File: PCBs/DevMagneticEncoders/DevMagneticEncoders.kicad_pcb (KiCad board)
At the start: 2 copper layers, 55 x 56 mm, 23 parts, among them J1 Conn_01x06_Male, J2 Conn_01x06_Male, J3 Screw_Terminal_01x02, J4 Conn_02x03_Odd_Even, J5 Conn_02x03_Odd_Even, J6 Conn_01x06_Male, J7 Conn_01x04_Male, J8 Conn_01x04_Male, U1 AZ1117-3.3, U2 ESP32-S2-WROOM

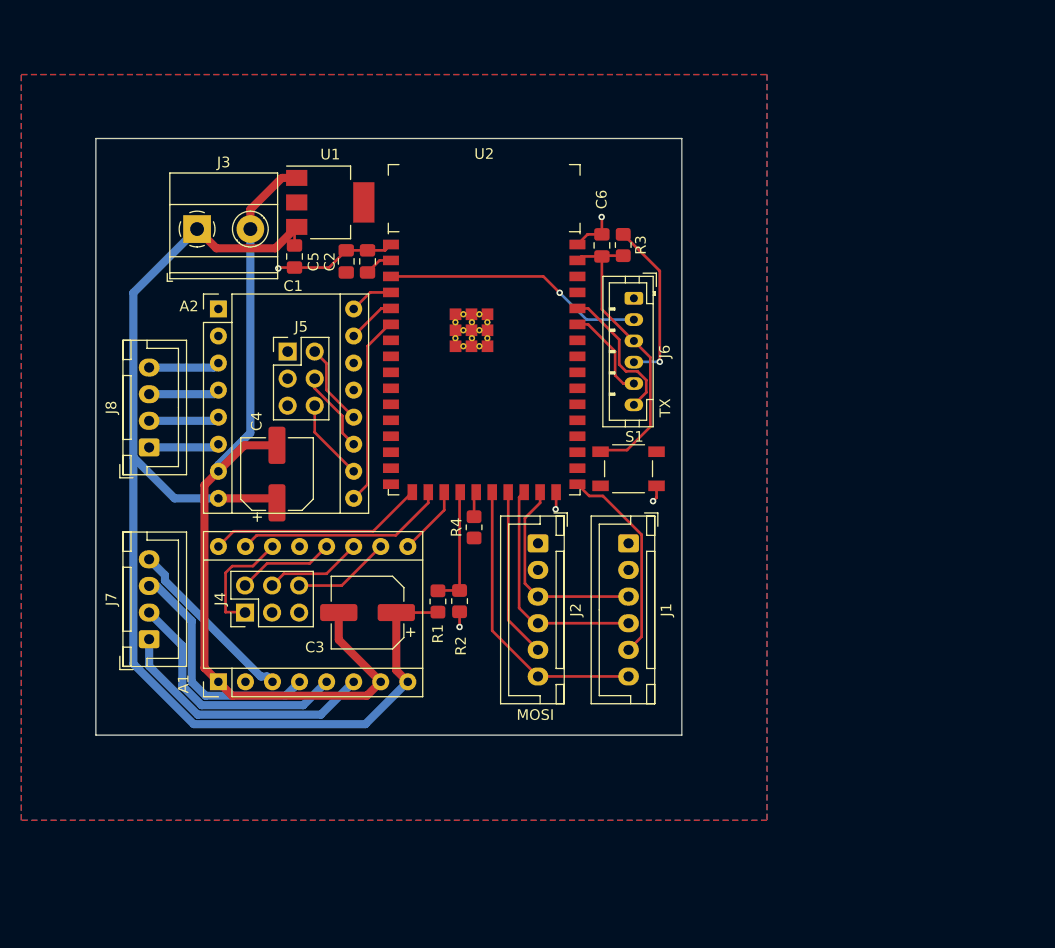
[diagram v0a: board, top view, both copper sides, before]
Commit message: 5 stepper board
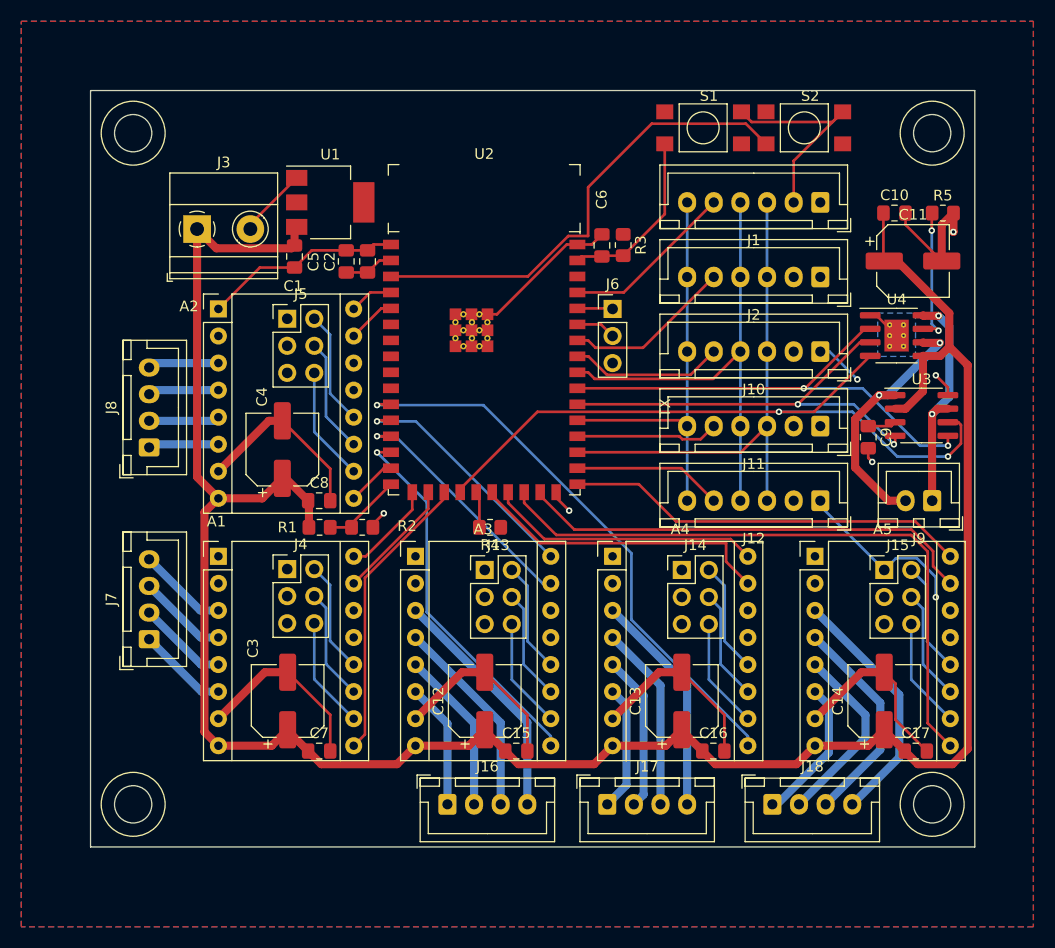
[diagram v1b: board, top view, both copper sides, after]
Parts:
- added A3: Pololu_Breakout_DRV8825, Module:Pololu_Breakout-16_15.2x20.3mm, F.Cu at (92.0, 95.2)
- added A4: Pololu_Breakout_DRV8825, Module:Pololu_Breakout-16_15.2x20.3mm, F.Cu at (110.5, 95.2)
- added A5: Pololu_Breakout_DRV8825, Module:Pololu_Breakout-16_15.2x20.3mm, F.Cu at (129.5, 95.2)
- added C10: 0.1U, Capacitor_SMD:C_0805_2012Metric_Pad1.18x1.45mm_HandSolder, F.Cu at (137.0, 63.0)
- added C11: 100U, Capacitor_SMD:CP_Elec_6.3x7.7, F.Cu at (138.7, 67.5)
- added C12: 100u, Capacitor_SMD:CP_Elec_6.3x7.7, F.Cu at (98.5, 108.8)
- added C13: 100u, Capacitor_SMD:CP_Elec_6.3x7.7, F.Cu at (117.0, 108.8)
- added C14: 100u, Capacitor_SMD:CP_Elec_6.3x7.7, F.Cu at (136.0, 108.8)
- added C15: 0.1u, Capacitor_SMD:C_0805_2012Metric_Pad1.18x1.45mm_HandSolder, F.Cu at (101.5, 113.5)
- added C16: 0.1u, Capacitor_SMD:C_0805_2012Metric_Pad1.18x1.45mm_HandSolder, F.Cu at (120.0, 113.5)
- added C17: 0.1u, Capacitor_SMD:C_0805_2012Metric_Pad1.18x1.45mm_HandSolder, F.Cu at (139.0, 113.5)
- added C7: 0.1u, Capacitor_SMD:C_0805_2012Metric_Pad1.18x1.45mm_HandSolder, F.Cu at (83.0, 113.5)
- added C8: 0.1u, Capacitor_SMD:C_0805_2012Metric_Pad1.18x1.45mm_HandSolder, F.Cu at (83.0, 90.0)
- added C9: 1U, Capacitor_SMD:C_0805_2012Metric_Pad1.18x1.45mm_HandSolder, F.Cu at (134.5, 84.0)
- added J10: Conn_01x06_Male, Connector_JST:JST_XH_B6B-XH-A_1x06_P2.50mm_Vertical, F.Cu at (130.0, 76.0)
- added J11: Conn_01x06_Male, Connector_JST:JST_XH_B6B-XH-A_1x06_P2.50mm_Vertical, F.Cu at (130.0, 83.0)
- added J12: Conn_01x06_Male, Connector_JST:JST_XH_B6B-XH-A_1x06_P2.50mm_Vertical, F.Cu at (130.0, 90.0)
- added J13: Conn_02x03_Odd_Even, Connector_PinHeader_2.54mm:PinHeader_2x03_P2.54mm_Vertical, F.Cu at (98.5, 96.5)
- added J14: Conn_02x03_Odd_Even, Connector_PinHeader_2.54mm:PinHeader_2x03_P2.54mm_Vertical, F.Cu at (117.0, 96.5)
- added J15: Conn_02x03_Odd_Even, Connector_PinHeader_2.54mm:PinHeader_2x03_P2.54mm_Vertical, F.Cu at (136.0, 96.5)
- added J16: Conn_01x04_Male, Connector_JST:JST_XH_B4B-XH-A_1x04_P2.50mm_Vertical, F.Cu at (95.0, 118.5)
- added J17: Conn_01x04_Male, Connector_JST:JST_XH_B4B-XH-A_1x04_P2.50mm_Vertical, F.Cu at (110.0, 118.5)
- added J18: Conn_01x04_Male, Connector_JST:JST_XH_B4B-XH-A_1x04_P2.50mm_Vertical, F.Cu at (125.5, 118.5)
- added J9: Conn_01x02_Male, Connector_JST:JST_XH_B2B-XH-A_1x02_P2.50mm_Vertical, F.Cu at (140.5, 90.0)
- added R5: 0.1, Resistor_SMD:R_0805_2012Metric_Pad1.20x1.40mm_HandSolder, F.Cu at (141.5, 63.0)
- added S2: TL3315NF160Q, A4:TL3305AF160QG, F.Cu at (128.5, 55.0)
- added U3: ZXBM5210-S, Package_SO:SOIC-8_3.9x4.9mm_P1.27mm, F.Cu at (139.5, 82.0)
- added U4: TB67H451FNG,EL, Package_SO:SOIC-8-1EP_3.9x4.9mm_P1.27mm_EP2.29x3mm_ThermalVias, F.Cu at (137.2, 74.5)
- J6: value Conn_01x06_Male -> Conn_01x03_Male; footprint Connector_JST:JST_PH_B6B-PH-K_1x06_P2.00mm_Vertical -> Connector_PinHeader_2.54mm:PinHeader_1x03_P2.54mm_Vertical
- S1: footprint A4:CK_PTS647_4.5x4.5 -> A4:TL3305AF160QG
- moved J1 36.7 mm to (130.0, 62.0), turned to 180 degrees
- moved J2 36.4 mm to (130.0, 69.0), turned to 180 degrees
- moved S1 32.8 mm to (119.0, 55.0)
- moved R1 13.1 mm to (83.0, 92.5), turned to 0 degrees
- moved A1 11.8 mm to (73.5, 95.2), turned to 0 degrees
- moved R2 11.5 mm to (87.0, 92.5), turned to 0 degrees
- moved C3 11.2 mm to (80.0, 108.8), turned to 90 degrees
- moved J4 5.69 mm to (80.0, 96.4), turned to 0 degrees
- moved J5 3.08 mm to (80.0, 72.9)
- moved C4 2.35 mm to (79.5, 85.2)
- moved J6 2.24 mm to (110.5, 72.0), turned to 0 degrees
- moved R4 1.50 mm to (99.0, 92.5), turned to 180 degrees
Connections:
- J6 pad 1: GND -> TX
- J6 pad 2: IO0 -> RX
- J6 pad 3: EN -> GND
- U2 pad 11: Net-(U2-Pad11) -> EN3
- U2 pad 12: Net-(U2-Pad12) -> DIR2
- U2 pad 13: Net-(U2-Pad13) -> STEP2
- U2 pad 14: Net-(U2-Pad14) -> EN2
- U2 pad 15: Net-(U2-Pad15) -> EN1
- U2 pad 16: Net-(U2-Pad16) -> CHARGE
- U2 pad 20: CHARGE -> DAC1
- U2 pad 22: MOSI -> STEP3
- U2 pad 23: CS1 -> DIR3
- U2 pad 24: MISO -> EN4
- U2 pad 25: CLK -> STEP4
- U2 pad 27: CS0 -> DIR4
- U2 pad 28: Net-(U2-Pad28) -> CS4
- U2 pad 29: Net-(U2-Pad29) -> CLK
- U2 pad 30: Net-(U2-Pad30) -> CS3
- U2 pad 31: Net-(U2-Pad31) -> MOSI
- U2 pad 32: Net-(U2-Pad32) -> MOT1
- U2 pad 33: Net-(U2-Pad33) -> MOT2
- U2 pad 34: Net-(U2-Pad34) -> MISO
- U2 pad 35: Net-(U2-Pad35) -> CS2
- U2 pad 36: Net-(U2-Pad36) -> CS1
- U2 pad 39: Net-(U2-Pad39) -> CS0
- U2 pad 6: EN1 -> Net-(U2-Pad6)
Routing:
- net +12V: track 111.9 -> 220.1 mm
- net GND: track 121.7 -> 192.8 mm
- net DAC1: track 0.00 -> 66.4 mm, vias 0 -> 2
- net EN4: track 0.00 -> 59.9 mm
- net EN3: track 0.00 -> 53.6 mm, vias 0 -> 1
- net MOT2: track 0.00 -> 46.5 mm, vias 0 -> 2
- net STEP4: track 0.00 -> 43.0 mm
- net MOT1: track 0.00 -> 41.3 mm, vias 0 -> 2
- net DIR4: track 0.00 -> 37.8 mm
- net EN2: track 0.00 -> 35.6 mm, vias 0 -> 1
- net STEP3: track 0.00 -> 28.7 mm
- net CLK: track 19.4 -> 46.8 mm
- net DIR3: track 0.00 -> 25.6 mm
- net OUT1: track 0.00 -> 24.6 mm, vias 0 -> 2
- net STEP2: track 0.00 -> 23.3 mm, vias 0 -> 1
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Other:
- board size 55 x 56 mm -> 83 x 71 mm
- board text removed: "MOSI"
